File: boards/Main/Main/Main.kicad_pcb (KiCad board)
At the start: 2 copper layers, 76 x 92.5 mm, 29 parts, among them Q1 2N3904, Q2 2N3904, Q3 2N3904

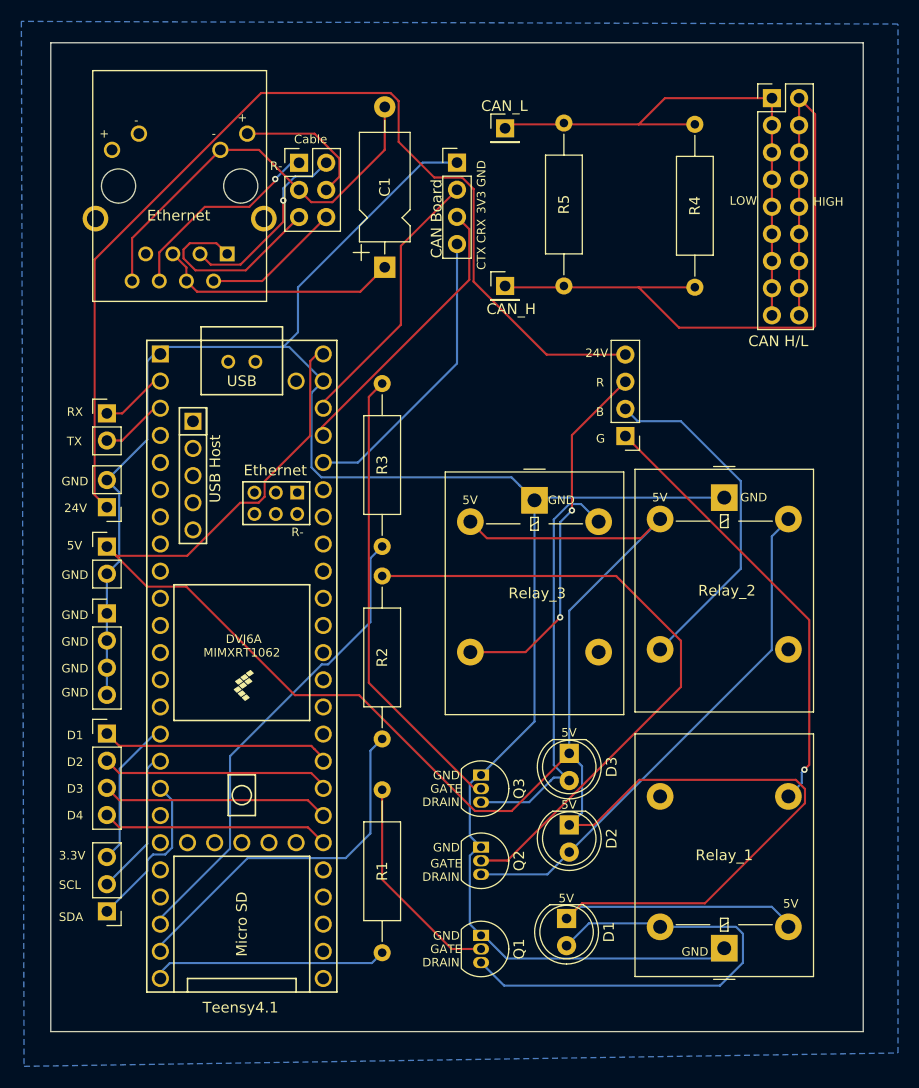
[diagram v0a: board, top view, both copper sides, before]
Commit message: Add files via upload
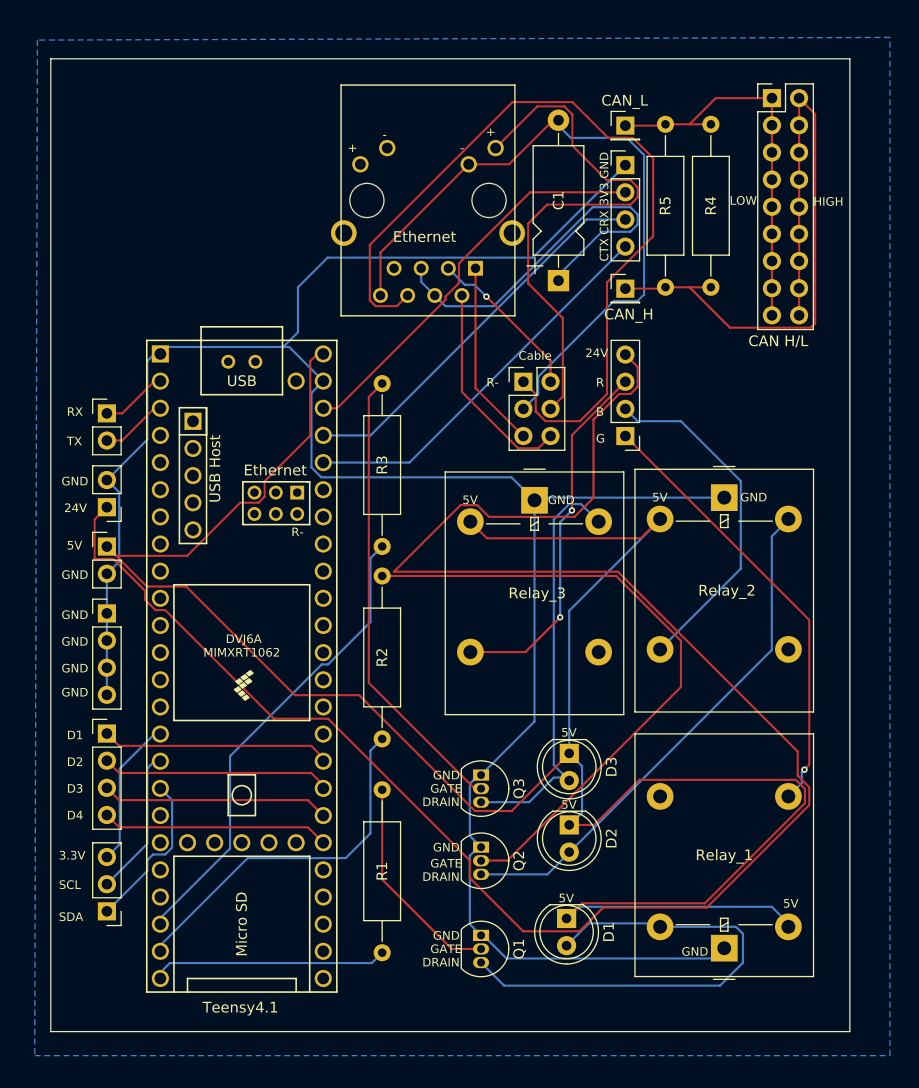
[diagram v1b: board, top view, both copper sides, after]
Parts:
- moved Ethernet_Cable1 29.3 mm to (135.7, 77.0)
- moved Ethernet1 23.3 mm to (126.8, 60.0)
- moved C1 16.3 mm to (139.0, 67.5)
- moved CAN_Board1 15.8 mm to (145.2, 56.7)
- moved CAN_H1 11.3 mm to (145.2, 68.2)
- moved CAN_L1 11.3 mm to (145.2, 53.0)
- moved R5 9.50 mm to (149.0, 52.9)
- moved R4 1.50 mm to (153.2, 68.1)
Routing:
- net +24V: track 97.2 -> 181.8 mm
- net Net-(Ethernet1-RD-): track 19.3 -> 78.8 mm, vias 1 -> 0
- net Net-(Ethernet1-LA): track 13.0 -> 51.1 mm
- net Net-(Ethernet1-GND): track 39.1 -> 64.9 mm
- net GND: track 197.4 -> 213.1 mm
- net /M1H: track 78.2 -> 63.5 mm
- net Net-(Ethernet1-CTR): track 23.0 -> 37.6 mm
- net /M1L: track 51.6 -> 37.5 mm
- net Net-(CAN_Board1-Pin_2): track 25.2 -> 37.9 mm
- net Net-(CAN_Board1-Pin_3): track 26.2 -> 37.0 mm
- net Net-(CAN_Board1-Pin_4): track 27.5 -> 36.6 mm
- net Net-(Ethernet1-TD-): track 13.0 -> 20.0 mm
- net Net-(Ethernet1-RD+): track 18.0 -> 15.1 mm
- net Net-(Ethernet1-TD+): track 18.9 -> 17.5 mm
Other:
- board size 76 x 92.5 mm -> 74.8 x 91 mm
- board text removed: "CAN Board"
